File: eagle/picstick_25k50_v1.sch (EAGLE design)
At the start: 16 parts, among them SW1 Reset, U1 PIC18F25K50-I/SP, X1 XTAL

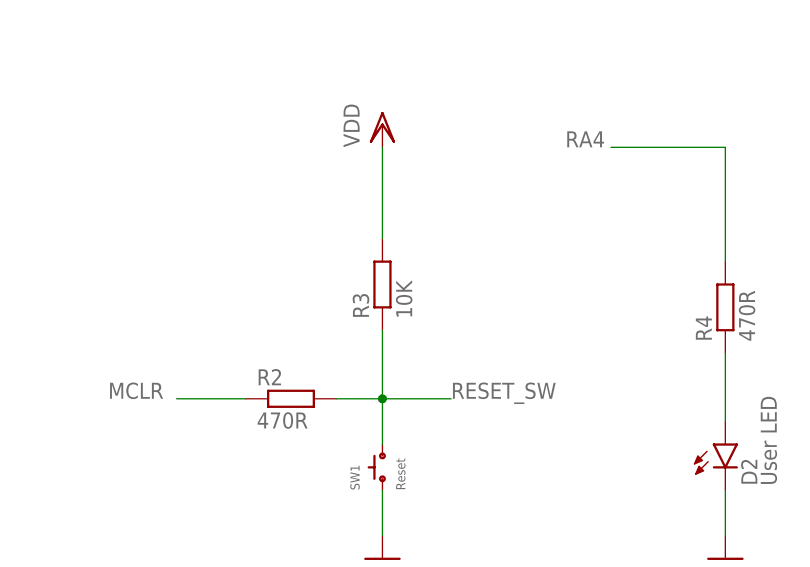
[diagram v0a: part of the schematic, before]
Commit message: ...
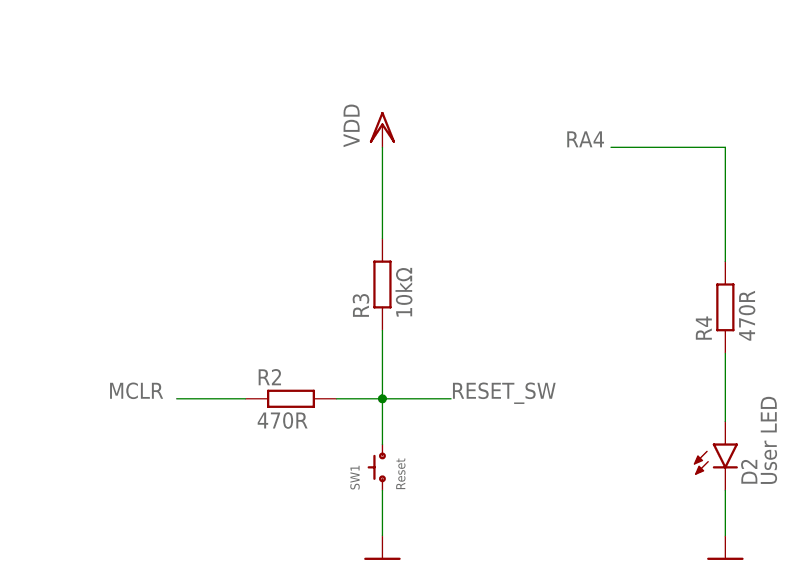
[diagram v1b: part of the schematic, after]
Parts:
- R3: value 10K -> 10kΩ
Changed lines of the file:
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@@
 <part name="GND2" library="LeoStick" deviceset="SUPPLY1_GND" device="" value=""/>
 <part name="R4" library="rcl" deviceset="R-EU_" device="0204/7" value="470R"/>
-<part name="R3" library="rcl" deviceset="R-EU_" device="0204/7" value="10K"/>
+<part name="R3" library="rcl" deviceset="R-EU_" device="0204/7" value="10kΩ" />
 <part name="R2" library="rcl" deviceset="R-EU_" device="0204/7" value="470R"/>
 <part name="GND4" library="LeoStick" deviceset="SUPPLY1_GND" device="" value=""/>

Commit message: ...
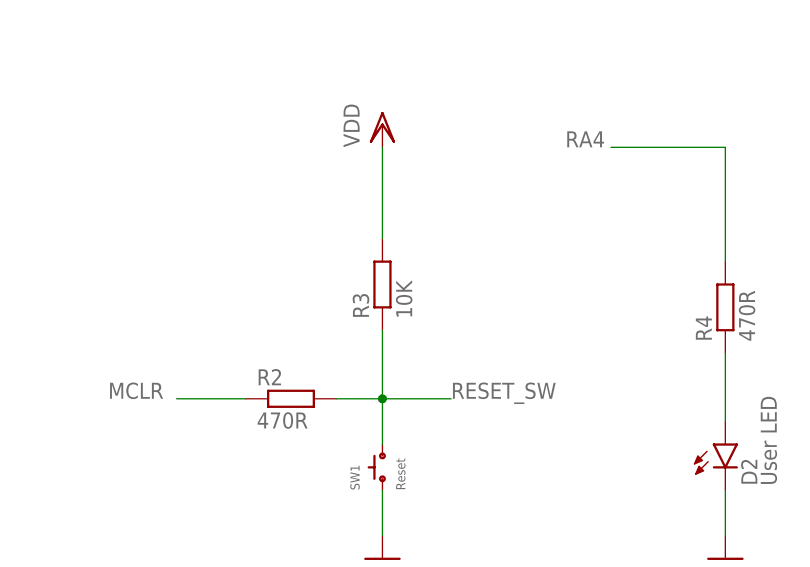
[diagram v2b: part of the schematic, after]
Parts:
- R3: value 10kΩ -> 10K
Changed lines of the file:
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@@
 <setting verticaltext="up"/>
 </settings>
-<grid distance="0.1" unitdist="inch" unit="inch" style="lines" multiple="1" display="yes" altdistance="2" altunitdist="inch" altunit="inch"/>
+<grid distance="0.05" unitdist="inch" unit="inch" style="lines" multiple="2" display="yes" altdistance="4" altunitdist="inch" altunit="inch"/>
 <layers>
 <layer number="1" name="Top" color="4" fill="1" visible="no" active="no"/>
@@
 <part name="GND2" library="LeoStick" deviceset="SUPPLY1_GND" device="" value=""/>
 <part name="R4" library="rcl" deviceset="R-EU_" device="0204/7" value="470R"/>
-<part name="R3" library="rcl" deviceset="R-EU_" device="0204/7" value="10kΩ" />
+<part name="R3" library="rcl" deviceset="R-EU_" device="0204/7" value="10K"/>
 <part name="R2" library="rcl" deviceset="R-EU_" device="0204/7" value="470R"/>
 <part name="GND4" library="LeoStick" deviceset="SUPPLY1_GND" device="" value=""/>

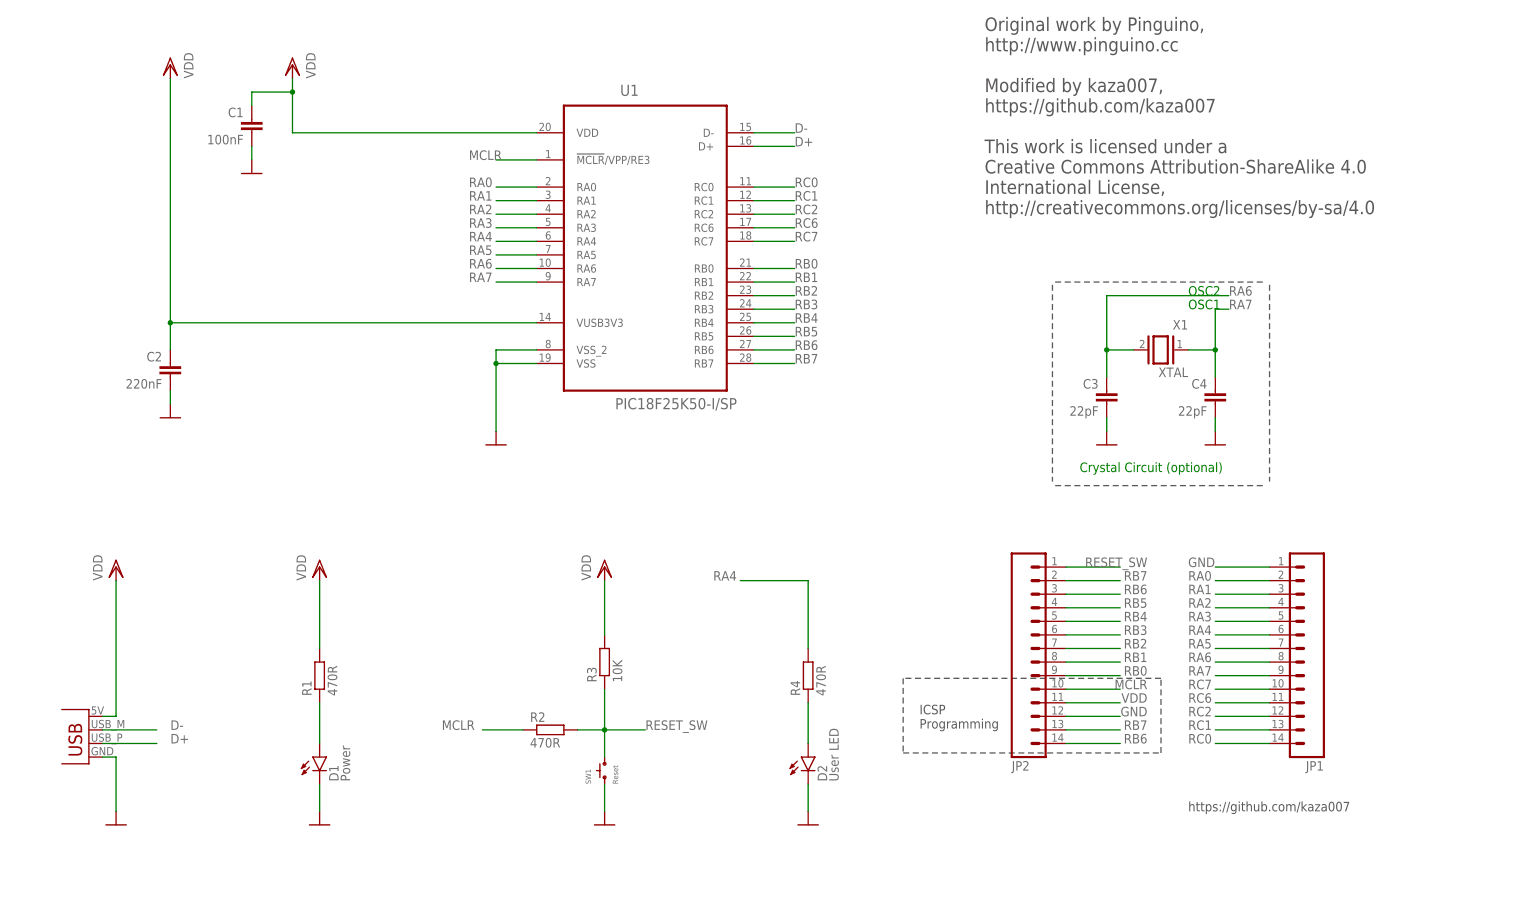
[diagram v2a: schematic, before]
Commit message: ...
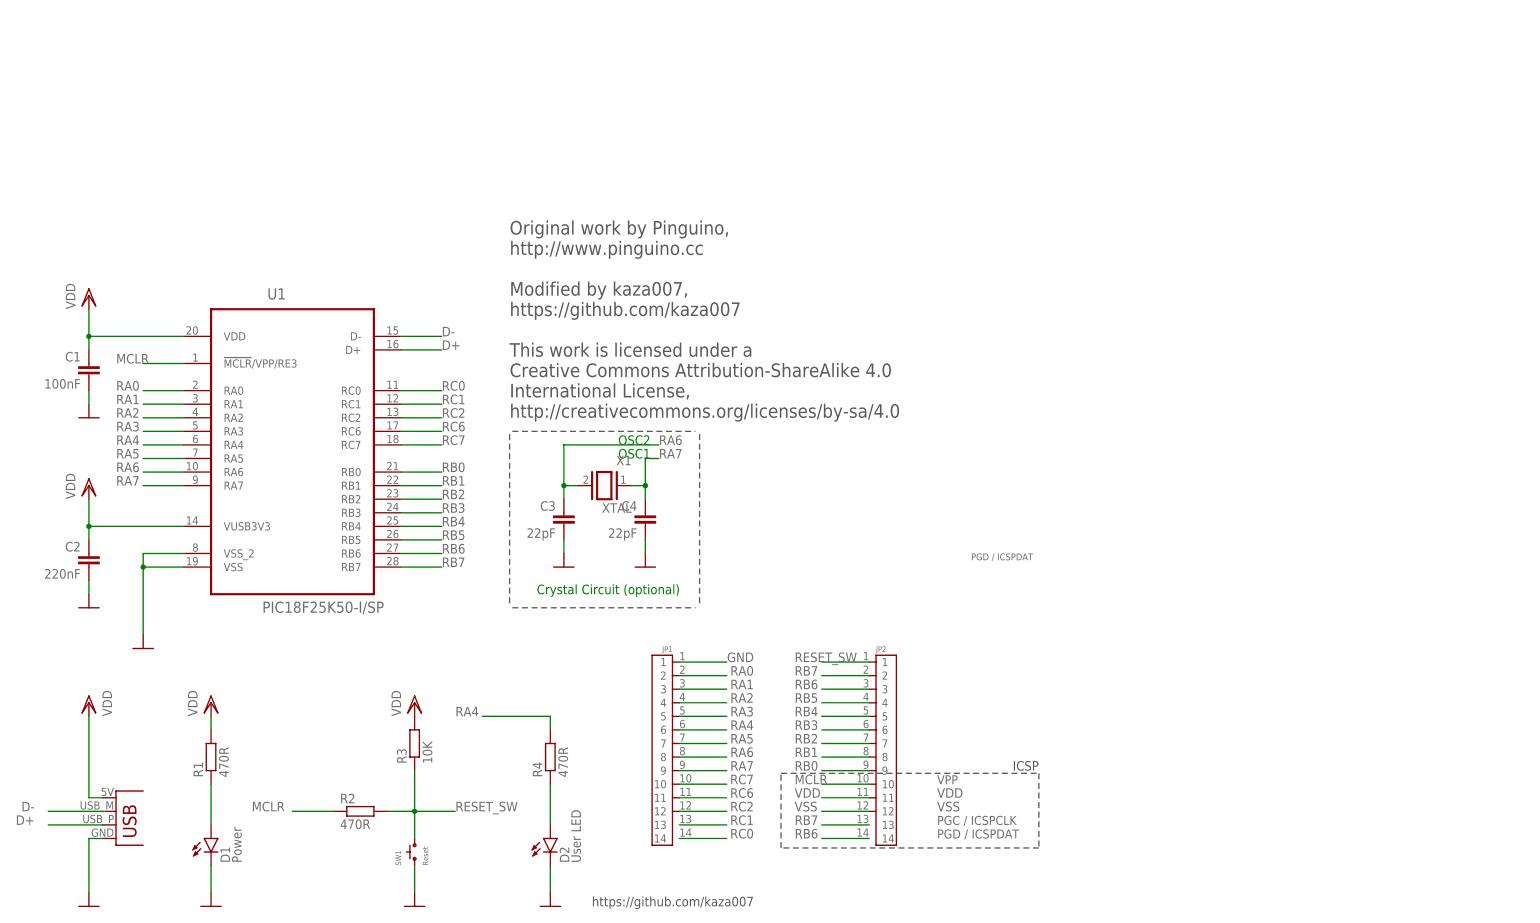
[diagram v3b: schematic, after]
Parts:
- JP1, JP2: value FREETRONICS-JON_M14 -> CONN-14P; device LeoStick:FREETRONICS-JON_M14 -> pinconn:CONN-14P
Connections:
- new net VSS: JP2.12
- net GND: no longer JP2.12
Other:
- note added: "ICSP"
- note added: "PGC / ICSPCLK"
- note added: "PGD / ICSPDAT"
- note added: "VPP"
- note removed: "ICSP Programming"
- moved on the sheet: C1, C2, C3, C4, D1, D2, R1, R2, R3, R4, SW1, U1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

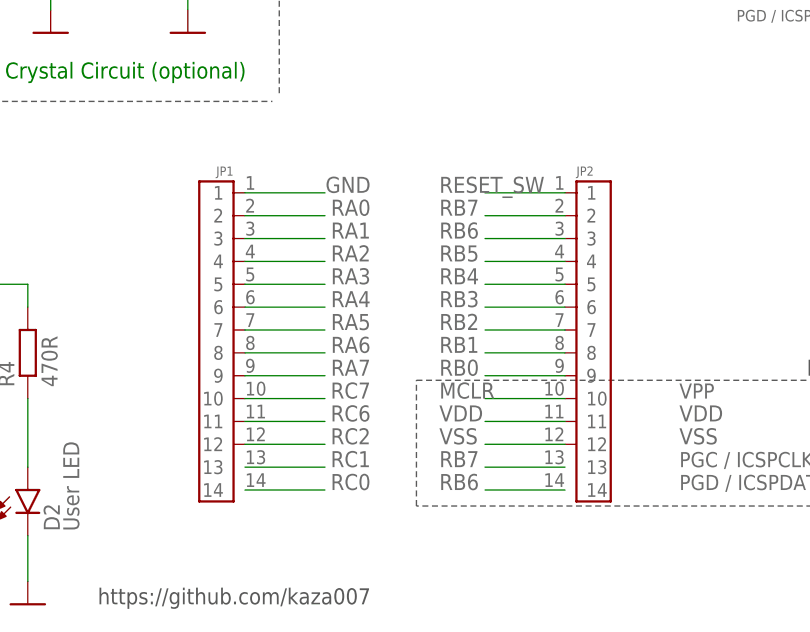
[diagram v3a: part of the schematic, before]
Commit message: ...
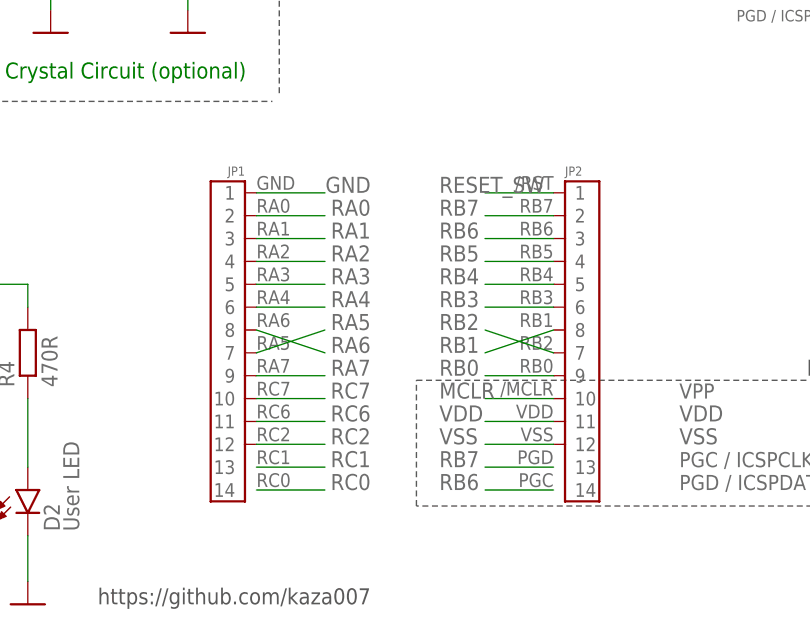
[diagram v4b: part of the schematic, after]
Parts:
- JP1: value CONN-14P -> CONN-14P-PICSTICK-JP1; device pinconn:CONN-14P -> pinconn:CONN-14P-PICSTICK-JP1
- JP2: value CONN-14P -> CONN-14P-PICSTICK-JP2; device pinconn:CONN-14P -> pinconn:CONN-14P-PICSTICK-JP2
